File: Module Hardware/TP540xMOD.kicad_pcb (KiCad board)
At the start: 2 copper layers, 18 x 12.2 mm, 13 parts, among them J1 Conn_01x01_Male, J2 Conn_01x01_Male, J3 Conn_01x01_Male, J4 Conn_01x01_Male, U1 TPS5403

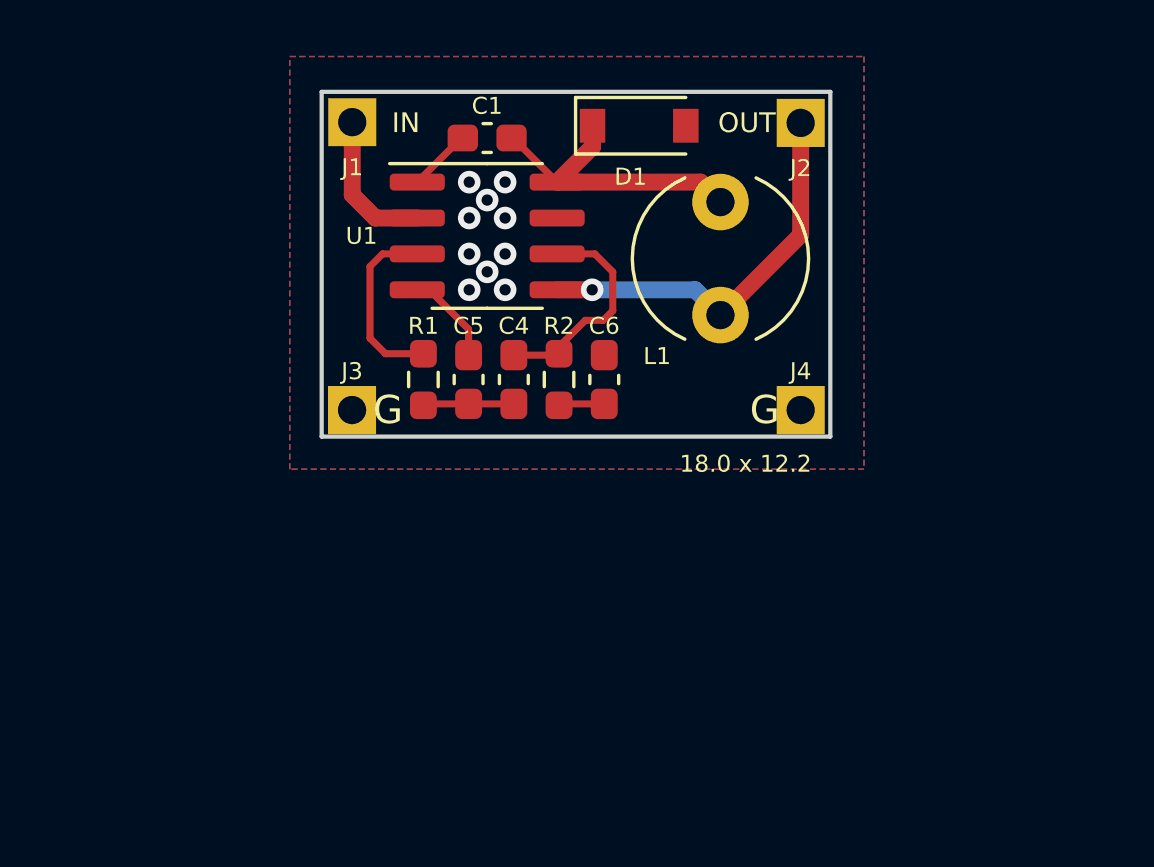
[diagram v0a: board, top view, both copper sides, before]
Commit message: ...
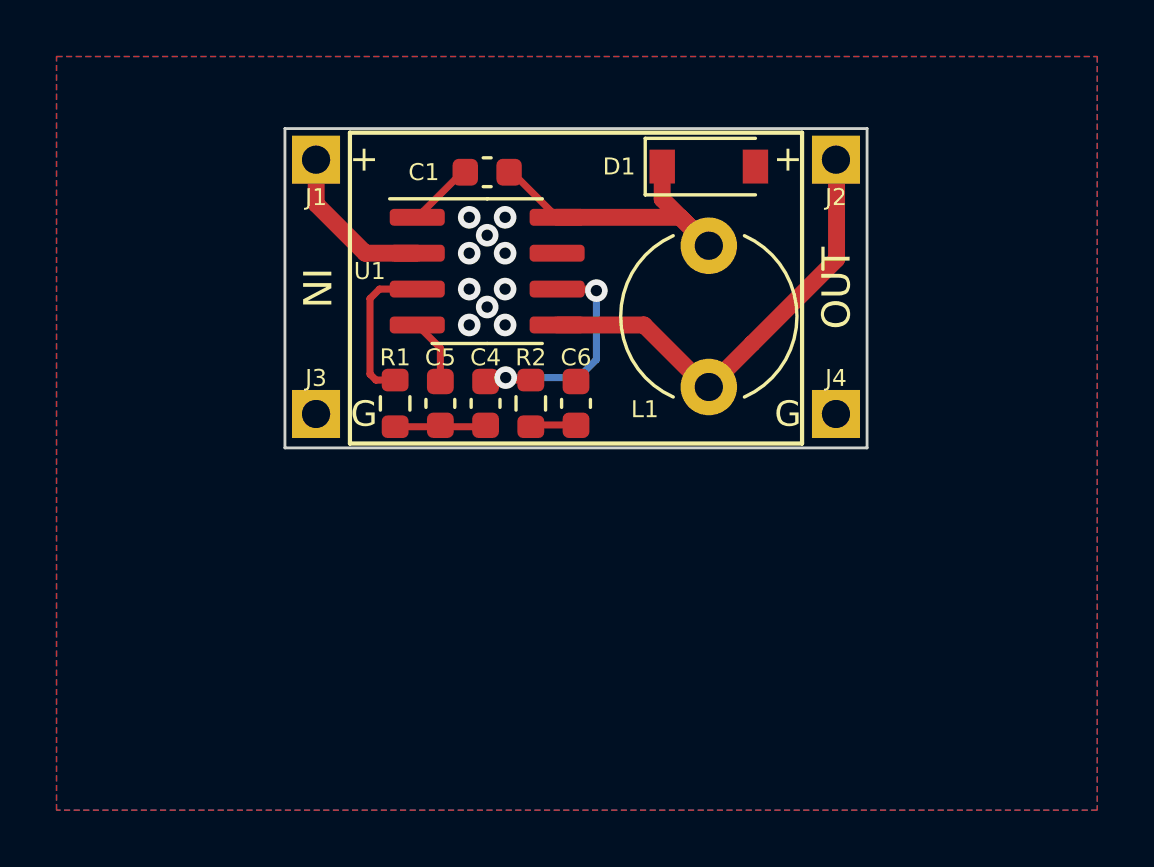
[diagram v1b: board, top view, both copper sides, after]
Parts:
- added REF**: DagNabbit, Tinker:DagNabbit, B.Cu at (92.7, 95.0)
- C1, C4, C5, C6: footprint Capacitor_SMD:C_0603_1608Metric_Pad1.08x0.95mm_HandSolder -> Capacitor_SMD:C_0603_1608Metric
- R1, R2: footprint Resistor_SMD:R_0603_1608Metric_Pad0.98x0.95mm_HandSolder -> Resistor_SMD:R_0603_1608Metric
- moved L1 4.07 mm to (104.7, 95.7)
- moved D1 2.86 mm to (104.7, 90.4)
- moved J1 1.85 mm to (90.8, 90.2)
- moved J2 1.80 mm to (109.2, 90.2)
- moved C4 1.31 mm to (96.8, 98.8)
- moved C5 1.31 mm to (95.2, 98.8)
- moved C6 1.31 mm to (100.0, 98.8)
- moved R1 1.31 mm to (93.6, 98.8)
- moved R2 1.31 mm to (98.4, 98.8)
- moved J3 1.28 mm to (90.8, 99.2)
- moved J4 1.26 mm to (109.2, 99.2)
- moved U1 1.24 mm to (96.9, 94.1)
- moved C1 1.21 mm to (96.9, 90.6)
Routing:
- net Vout: track 14.1 -> 16.2 mm, vias 1 -> 0
- net Net-(R1-Pad1): track 6.53 -> 5.46 mm
- net Net-(C4-Pad1): track 7.91 -> 8.95 mm, vias 0 -> 2
- net Net-(C5-Pad1): track 3.31 -> 2.34 mm
- net Net-(C1-Pad2): track 10.8 -> 11.5 mm
- net Vin: track 5.21 -> 5.90 mm
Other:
- board size 18 x 12.2 mm -> 20.6 x 11.3 mm
- board text added: "+"
- board text added: "S. A. Miller 2024"
- board text added: "TPS540x Carrier"
- board text removed: "18.0 x 12.2"
